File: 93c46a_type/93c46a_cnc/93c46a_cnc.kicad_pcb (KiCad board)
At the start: 2 copper layers, 38.7 x 36.8 mm, 17 parts, among them SW1 SW_SPST, U1 93CxxA, U2 74LS123, U4 NE555D

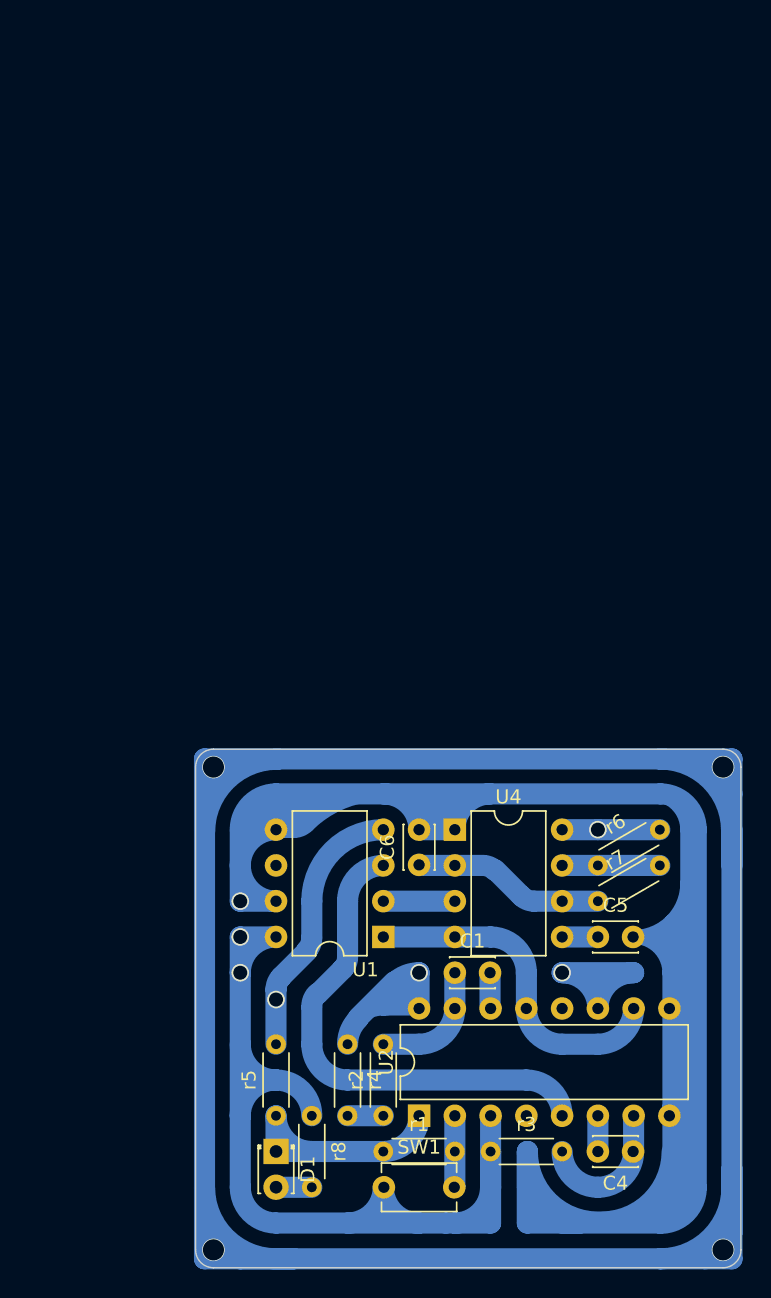
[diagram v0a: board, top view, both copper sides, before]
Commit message: pushing the way I know to use denford gcode plotter
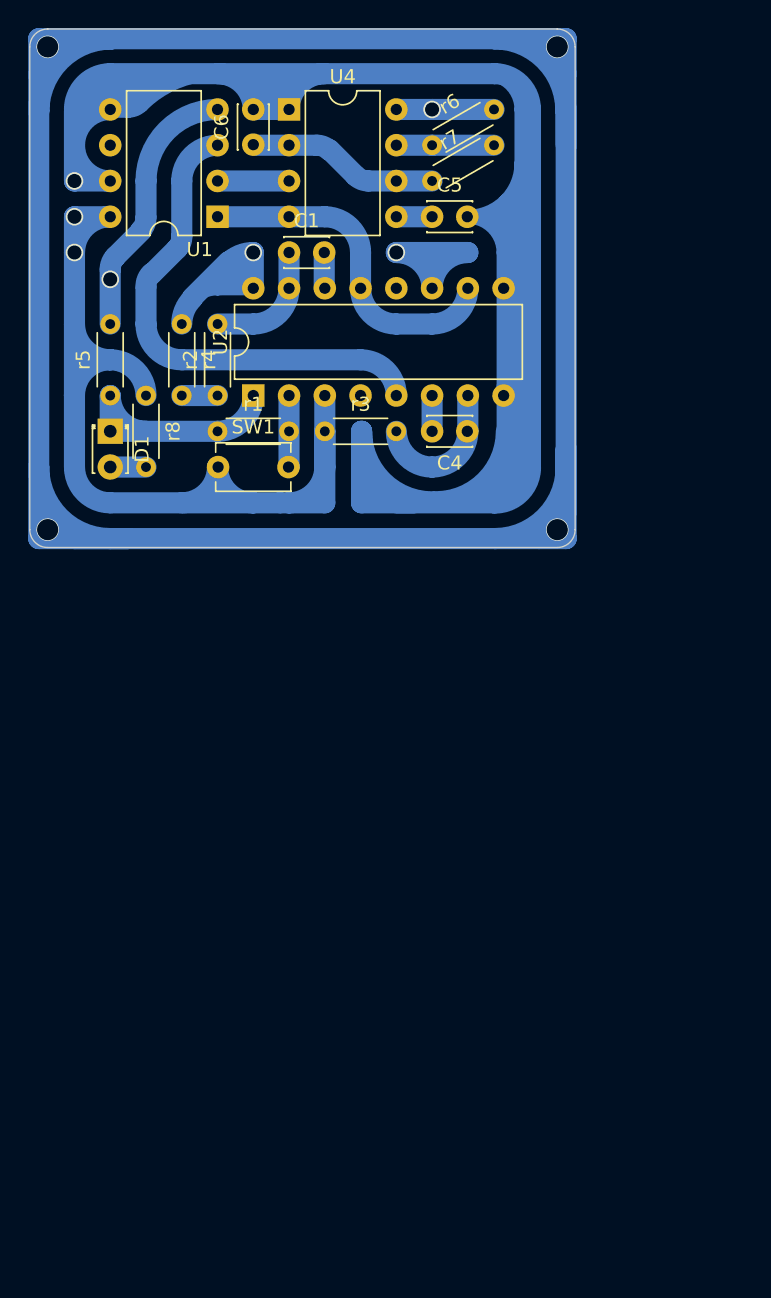
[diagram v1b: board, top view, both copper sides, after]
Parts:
- moved C1 52.5 mm to (19.4, -22.6)
- moved C4 52.5 mm to (32.0, -9.94)
- moved C5 52.5 mm to (29.5, -25.2)
- moved C6 52.5 mm to (16.8, -30.3)
- moved D1 52.5 mm to (6.67, -9.95)
- moved SW1 52.5 mm to (14.3, -7.40)
- moved U1 52.5 mm to (14.3, -25.2)
- moved U2 52.5 mm to (16.8, -12.5)
- moved r1 52.5 mm to (14.3, -9.94)
- moved r2 52.5 mm to (14.3, -12.5)
- moved r3 52.5 mm to (21.9, -9.94)
- moved r5 52.5 mm to (6.67, -12.5)
- moved r7 52.5 mm to (29.5, -27.7)
- moved r8 52.5 mm to (9.21, -12.5)
- moved U4 52.5 mm to (19.4, -32.8)
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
